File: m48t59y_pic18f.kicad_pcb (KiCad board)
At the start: 2 copper layers, 66 x 64.8 mm, 23 parts, among them J3 ssd1306, J4 Raspberry_Pi_4, U1 TXS0108, U2 TXS0108, U3 LM7805_TO220, U4 74HC595, U5 74HC595, U7 M48T08-150PC

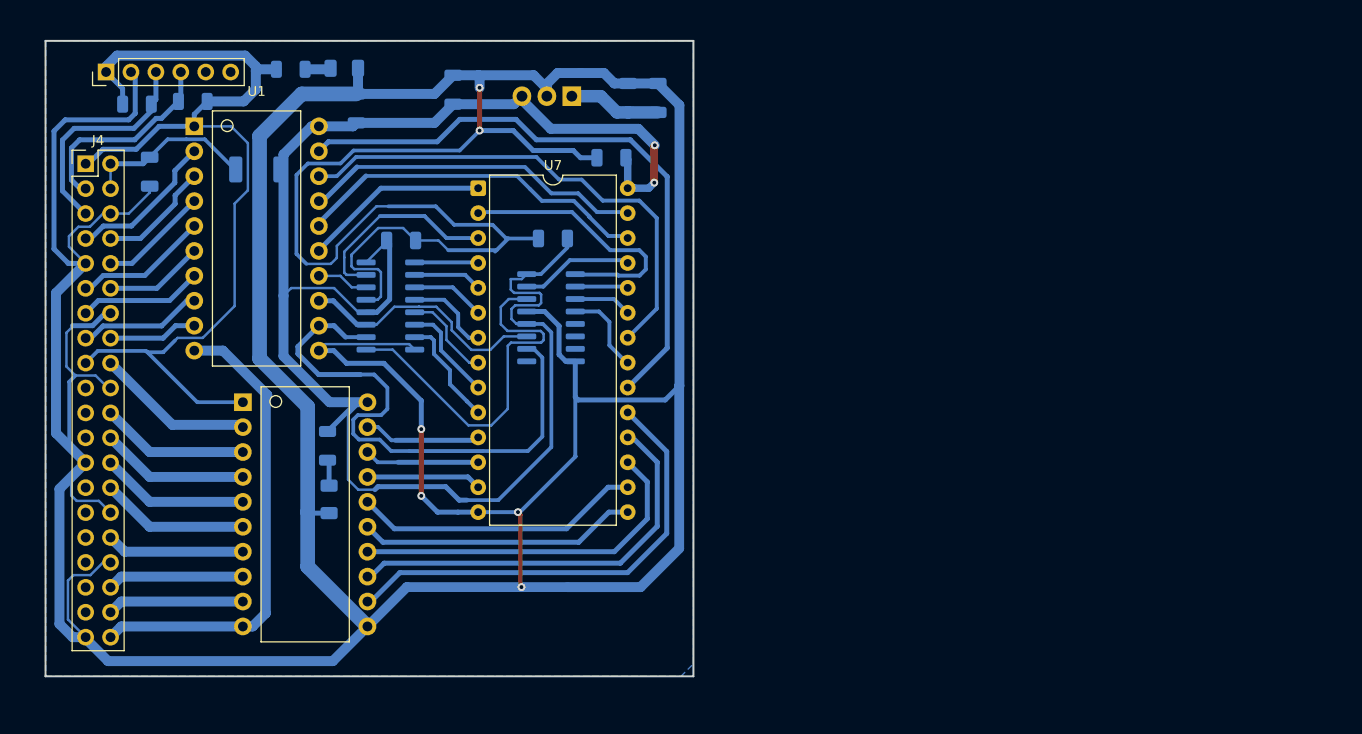
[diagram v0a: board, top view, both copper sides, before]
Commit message: Update schematics, PCB, and add fp-lib-table
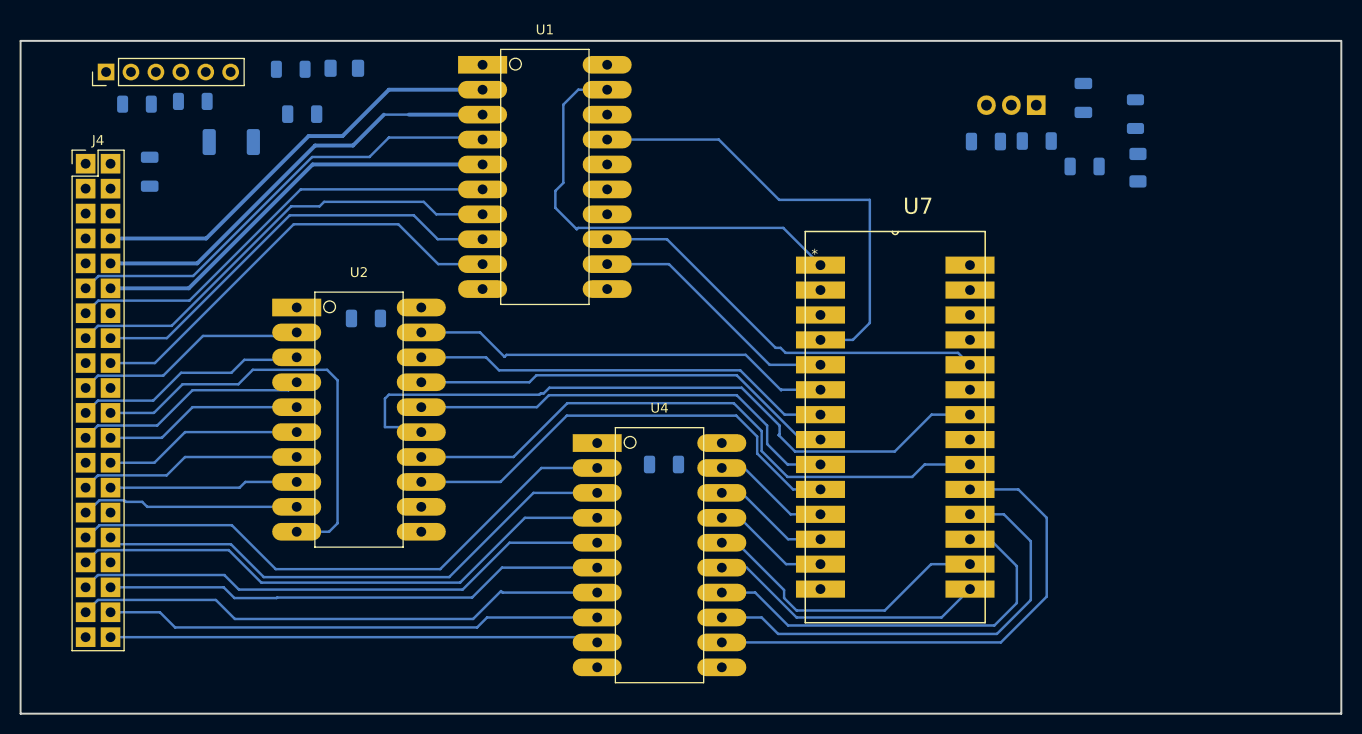
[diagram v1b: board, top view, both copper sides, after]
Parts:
- removed U5: 74HC595, Package_SO:SOIC-16_3.9x9.9mm_P1.27mm
- J4: footprint Connector_PinHeader_2.54mm:PinHeader_2x20_P2.54mm_Vertical -> kicad:PinHeader_2x20_P2.54mm_Vertical
- U1, U2: footprint kiC:TXS0108E_THT_20pin -> kicad:TXS0108E_THT_20pin_big
- U4: value 74HC595 -> TXS0108; footprint Package_SO:SOIC-16_3.9x9.9mm_P1.27mm -> kicad:TXS0108E_THT_20pin_big; moved to F.Cu
- U7: footprint Package_DIP:DIP-28_W15.24mm -> kicad:DIP-28_W15.24mm
- moved D1 89.1 mm to (207.9, 63.7)
- moved R11 89.0 mm to (207.6, 58.3)
- moved U7 64.7 mm to (190.8, 106.7)
- moved C6 54.7 mm to (202.4, 63.6)
- moved C5 54.6 mm to (192.4, 61.1), turned to 0 degrees
- moved U3 47.4 mm to (197.5, 57.4)
- moved C8 43.4 mm to (202.3, 56.6)
- moved C9 41.9 mm to (197.6, 61.0), turned to 180 degrees
- moved U4 37.4 mm to (159.1, 103.2), turned to 0 degrees
- moved C7 31.7 mm to (159.6, 94.0), turned to 0 degrees
- moved U1 30.1 mm to (147.4, 64.7)
- moved C4 21.4 mm to (129.2, 79.1), turned to 0 degrees
- moved C10 16.4 mm to (122.7, 58.3)
- moved U2 11.1 mm to (128.5, 89.4)
- moved D4 3.89 mm to (115.5, 61.1)
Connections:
- J4 pad 19: /RaspberryPi4/MOSI -> /RaspberryPi4/GPIO10
- J4 pad 21: /RaspberryPi4/MISO -> /RaspberryPi4/GPIO9
- J4 pad 23: /RaspberryPi4/SCLK -> /RaspberryPi4/GPIO11
- U1 pad 10: /RaspberryPi4/GPIO21 -> /RaspberryPi4/GPIO25
- U1 pad 12: /m48t59y/RCLK -> /m48t59y/A5
- U1 pad 13: /m48t59y/SRCCLK -> /m48t59y/A9
- U1 pad 14: /m48t59y/SER_IN -> /m48t59y/A8
- U1 pad 15: /m48t59y/INT -> /m48t59y/E2
- U1 pad 16: /m48t59y/E2 -> /m48t59y/W
- U1 pad 17: /m48t59y/W -> /m48t59y/A6
- U1 pad 18: /m48t59y/G -> /m48t59y/A7
- U1 pad 19: /m48t59y/E1 -> /m48t59y/INT
- U1 pad 2: /RaspberryPi4/GPIO4 -> /RaspberryPi4/GPIO14
- U1 pad 3: /RaspberryPi4/GPIO14 -> /RaspberryPi4/GPIO15
- U1 pad 4: /RaspberryPi4/GPIO15 -> /RaspberryPi4/GPIO17
- U1 pad 5: /RaspberryPi4/GPIO17 -> /RaspberryPi4/GPIO18
- U1 pad 6: /RaspberryPi4/GPIO18 -> /RaspberryPi4/GPIO27
- U1 pad 7: /RaspberryPi4/GPIO27 -> /RaspberryPi4/GPIO22
- U1 pad 8: /RaspberryPi4/GPIO22 -> /RaspberryPi4/GPIO23
- U1 pad 9: /RaspberryPi4/GPIO23 -> /RaspberryPi4/GPIO24
- U2 pad 10: /RaspberryPi4/GPIO21 -> /RaspberryPi4/GPIO25
- U2 pad 12: /m48t59y/DQ7 -> /txs0108e/B8B
- U2 pad 13: /m48t59y/DQ6 -> /m48t59y/A0
- U2 pad 14: /m48t59y/DQ5 -> /m48t59y/E1
- U2 pad 15: /m48t59y/DQ3 -> /m48t59y/G
- U2 pad 16: /m48t59y/DQ4 -> /m48t59y/A1
- U2 pad 17: /m48t59y/DQ2 -> /m48t59y/A2
- U2 pad 18: /m48t59y/DQ1 -> /m48t59y/A3
- U2 pad 19: /m48t59y/DQ0 -> /m48t59y/A4
- U2 pad 2: /RaspberryPi4/GPIO24 -> /RaspberryPi4/GPIO10
- U2 pad 3: /RaspberryPi4/GPIO25 -> /RaspberryPi4/GPIO9
- U2 pad 4: /RaspberryPi4/GPIO8 -> /RaspberryPi4/GPIO11
- U2 pad 5: /RaspberryPi4/GPIO7 -> /RaspberryPi4/GPIO8
- U2 pad 6: /RaspberryPi4/GPIO1 -> /RaspberryPi4/GPIO7
- U2 pad 7: /RaspberryPi4/GPIO12 -> /RaspberryPi4/GPIO0
- U2 pad 8: /RaspberryPi4/GPIO16 -> /RaspberryPi4/GPIO1
- U2 pad 9: /RaspberryPi4/GPIO20 -> /RaspberryPi4/GPIO5
- U4 pad 1: /m48t59y/Q1B -> +3V3
- U4 pad 10: /m48t59y/RCLK -> /RaspberryPi4/GPIO25
- U4 pad 11: /m48t59y/SRCCLK -> GND
- U4 pad 12: +5V -> /m48t59y/DQ7
- U4 pad 13: GND -> /m48t59y/DQ6
- U4 pad 14: /m48t59y/SER_IN -> /m48t59y/DQ5
- U4 pad 15: /m48t59y/Q1A -> /m48t59y/DQ3
- U4 pad 16: +5V -> /m48t59y/DQ4
- U4 pad 2: /m48t59y/Q1C -> /RaspberryPi4/GPIO6
- U4 pad 3: /m48t59y/Q1D -> /RaspberryPi4/GPIO12
- U4 pad 4: /m48t59y/Q1E -> /RaspberryPi4/GPIO13
- U4 pad 5: /m48t59y/Q1F -> /RaspberryPi4/GPIO19
- U4 pad 6: /m48t59y/Q1G -> /RaspberryPi4/GPIO16
- U4 pad 7: /m48t59y/Q1H -> /RaspberryPi4/GPIO26
- U4 pad 8: GND -> /RaspberryPi4/GPIO20
- U4 pad 9: Net-(U4-QH') -> /RaspberryPi4/GPIO21
- U7 pad 10: /m48t59y/Q1H -> /m48t59y/A0
- U7 pad 2: /m48t59y/Q2B -> /m48t59y/A12
- U7 pad 21: /m48t59y/Q2E -> /m48t59y/A10
- U7 pad 23: /m48t59y/Q2D -> /m48t59y/A11
- U7 pad 24: /m48t59y/Q2C -> /m48t59y/A9
- U7 pad 25: Net-(U5-QA) -> /m48t59y/A8
- U7 pad 3: /m48t59y/Q1A -> /m48t59y/A7
- U7 pad 4: /m48t59y/Q1B -> /m48t59y/A6
- U7 pad 5: /m48t59y/Q1C -> /m48t59y/A5
- U7 pad 6: /m48t59y/Q1D -> /m48t59y/A4
- U7 pad 7: /m48t59y/Q1E -> /m48t59y/A3
- U7 pad 8: /m48t59y/Q1F -> /m48t59y/A2
- U7 pad 9: /m48t59y/Q1G -> /m48t59y/A1
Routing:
- net GND: track 546.5 -> 0.00 mm, vias 6 -> 0
- net +5V: track 178.7 -> 0.00 mm, vias 2 -> 0
- net +3V3: track 99.3 -> 0.00 mm
- net /RaspberryPi4/GPIO6: track 0.00 -> 58.8 mm
- net /m48t59y/RCLK: track 58.3 -> 0.00 mm
- net /RaspberryPi4/GPIO13: track 0.00 -> 56.8 mm
- net /RaspberryPi4/GPIO19: track 0.00 -> 55.3 mm
- net /RaspberryPi4/GPIO26: track 0.00 -> 54.7 mm
- net /m48t59y/A0: track 0.00 -> 47.6 mm
- net /m48t59y/A6: track 0.00 -> 47.6 mm
- net /m48t59y/A1: track 0.00 -> 45.2 mm
- net /m48t59y/A2: track 0.00 -> 43.7 mm
- net /m48t59y/A4: track 0.00 -> 43.3 mm
- net /m48t59y/A3: track 0.00 -> 43.1 mm
- net /m48t59y/A9: track 0.00 -> 42.3 mm
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- removed copper zone on B.Cu, net GND
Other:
- board size 66 x 64.8 mm -> 134.6 x 68.6 mm
